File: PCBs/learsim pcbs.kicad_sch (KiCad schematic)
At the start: 54 parts, among them SW1 MHz, SW2 KHz, SW3 2MS1T1B1M2QES-5, U1 ESP32-C6-DEV-KIT-N8, U2 MAX7219, U3 MAX7219

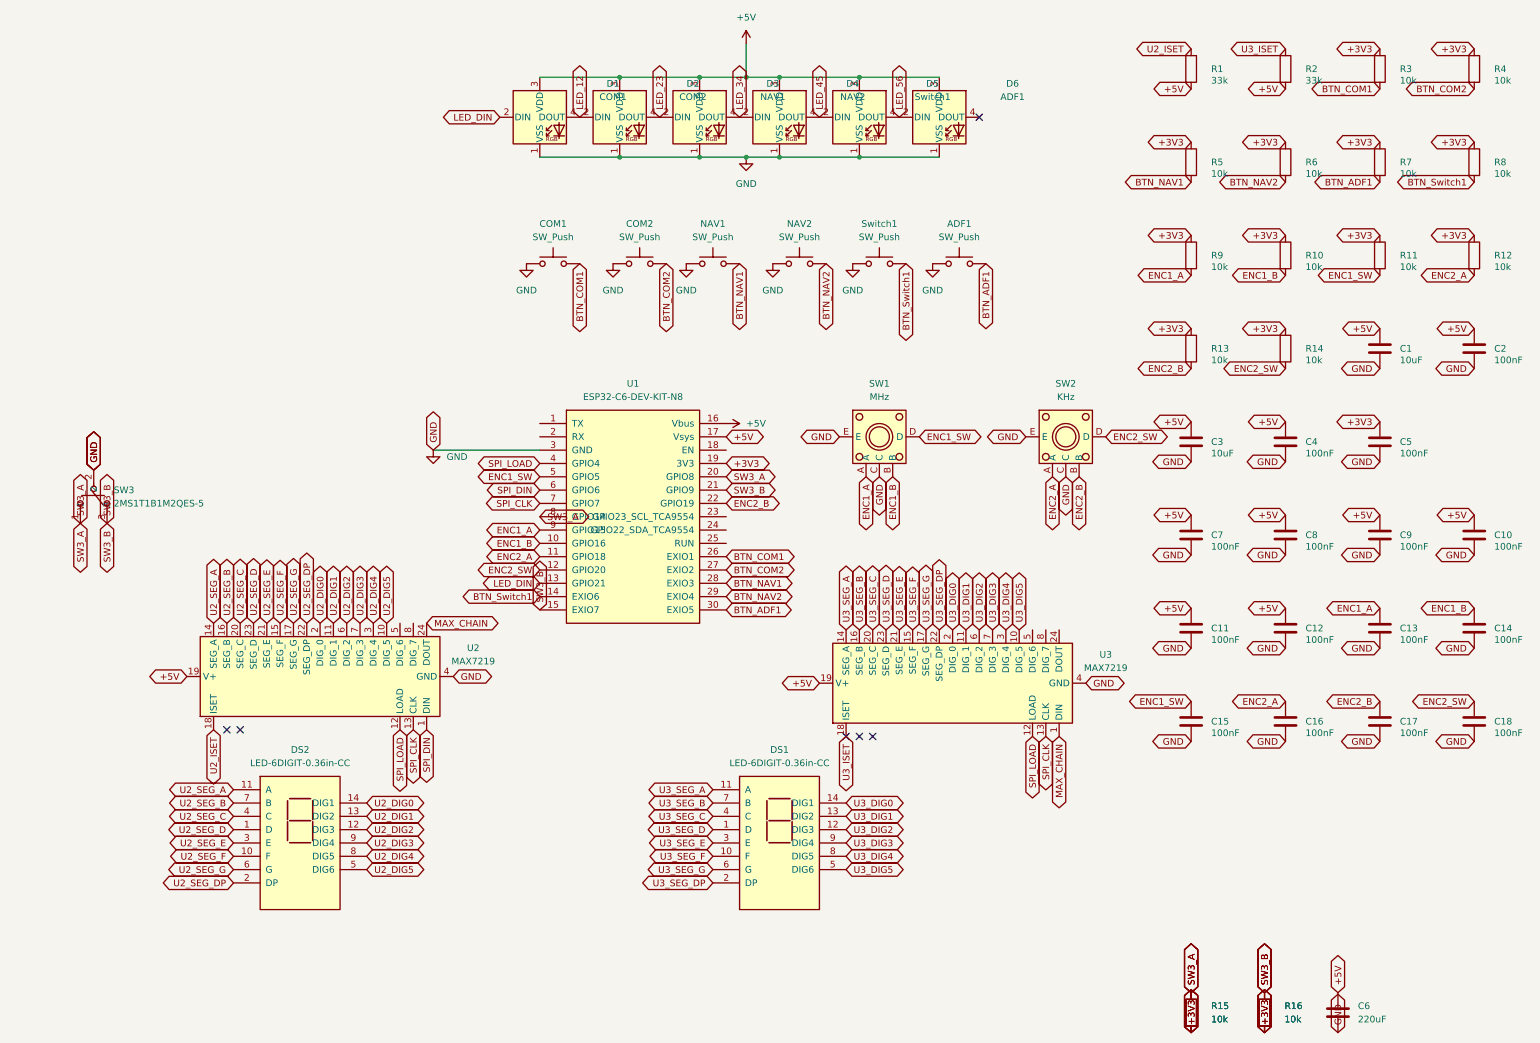
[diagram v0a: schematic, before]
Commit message: Refactor code structure for improved readability and maintainability
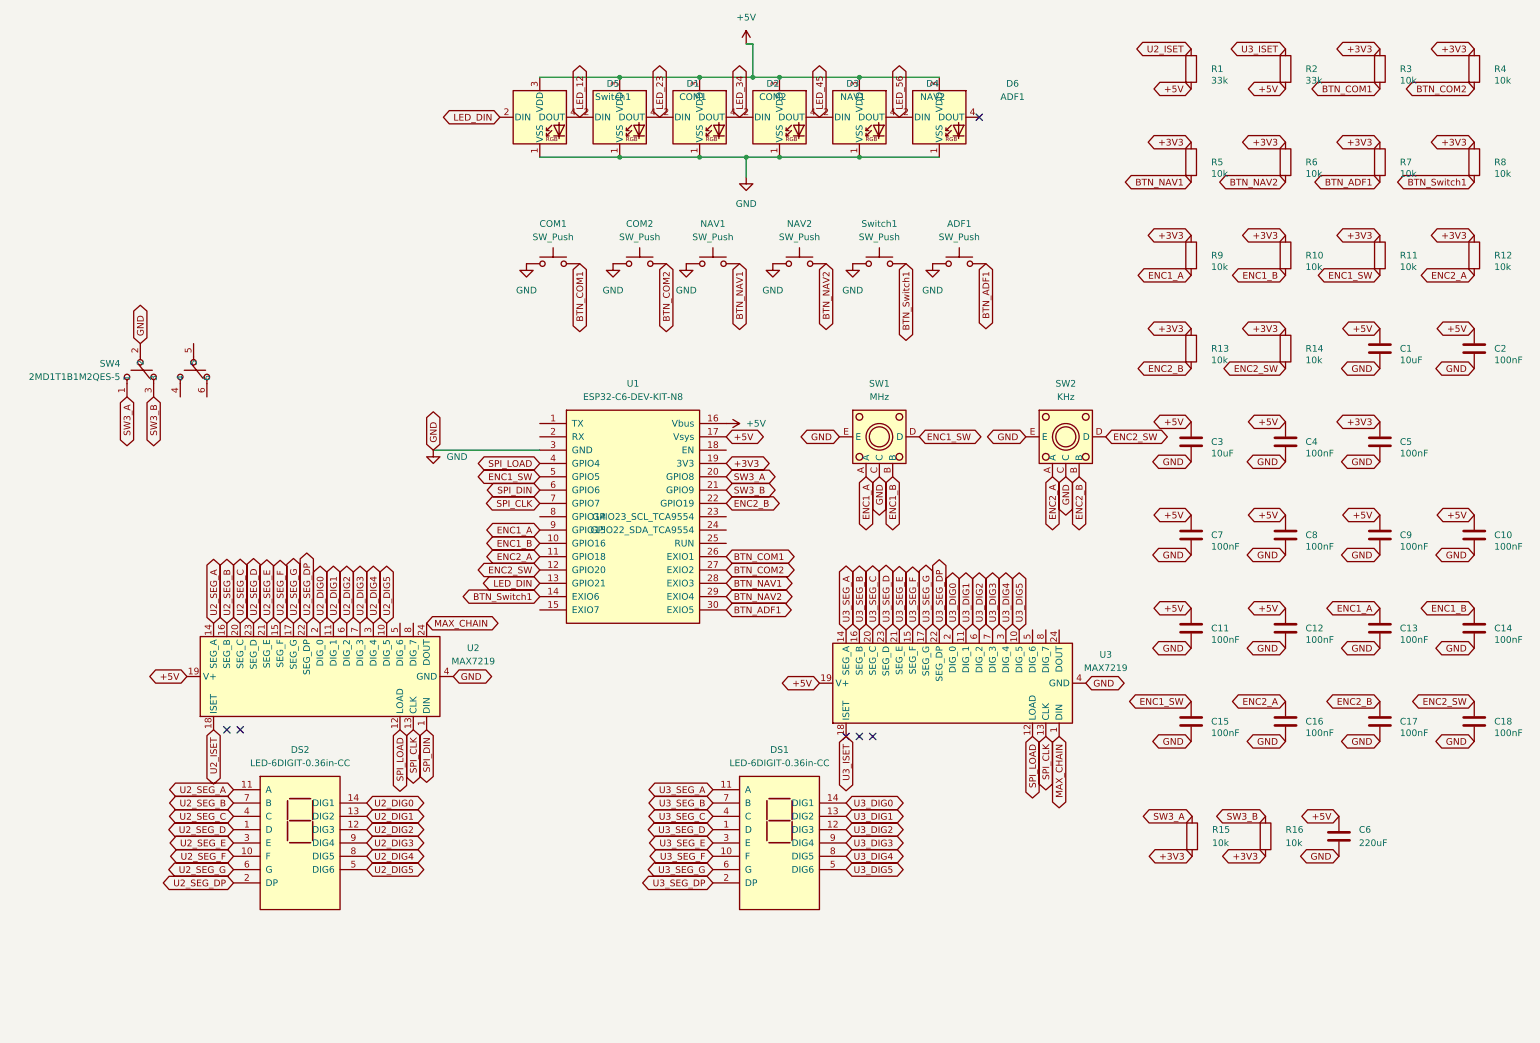
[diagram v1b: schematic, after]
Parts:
- removed SW3: 2MS1T1B1M2QES-5, Rotary:SW-TH_2MS1T1B1M2QES-5, symbol Rotary:2MS1T1B1M2QES-5
- added SW4: 2MD1T1B1M2QES-5, Rotary:SW-TH_2MD1T1B1M2QES-5, symbol Rotary:2MD1T1B1M2QES-5
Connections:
- net GND: now also SW4.2
- net LED_12: now also D1.2 (DIN), D5.4 (DOUT); no longer D1.4 (DOUT), D2.2 (DIN)
- net LED_23: now also D1.4 (DOUT), D2.2 (DIN); no longer D2.4 (DOUT), D3.2 (DIN)
- net LED_34: now also D2.4 (DOUT), D3.2 (DIN); no longer D3.4 (DOUT), D4.2 (DIN)
- net LED_45: now also D3.4 (DOUT), D4.2 (DIN); no longer D4.4 (DOUT), D5.2 (DIN)
- net LED_56: now also D4.4 (DOUT); no longer D5.4 (DOUT)
- net LED_DIN: now also D5.2 (DIN); no longer D1.2 (DIN)
- net SW3_A: now also SW4.1; no longer U1.8 (GPIO14)
- net SW3_B: now also SW4.3; no longer U1.15 (EXIO7)
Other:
- moved on the sheet: C6, D1, D2, D3, D4
